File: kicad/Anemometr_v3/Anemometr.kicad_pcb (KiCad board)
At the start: 2 copper layers, 45 x 45 mm, 170 parts, among them J1 TxD, J10 +Z1, J11 +Z2, J12 +Z3, J13 +Z4, J14 -Z1, J15 -Z2, J16 -Z3, J17 -Z4, J18 1 TxD+, J19 2 TxD-, J2 RxD, J20 3 RxD+, J21 4-5, J22 6 RxD-, J23 7-8, J24 Conn_01x01_Female, J25 Conn_01x01_Female, J26 Conn_01x01_Female, J3 SCL, J4 SDA, J5 RST, J6 +EXT, J7 -EXT, J8 SWD, J9 SWC, Q1 5N10, U1 STM32F103C8Tx, U2 TS5A3166DBVR, U3 TS5A3166DBVR, U4 LMR14206, U5 TS5A3166DBVR, U6 NCP1117-3.3, U7 TS5A3166DBVR, U8 MCP1703-3.3, U9 MCP1703-3.3, Y1 CSTCE8M00G52A-R0, Y2 ECS-250-20-33

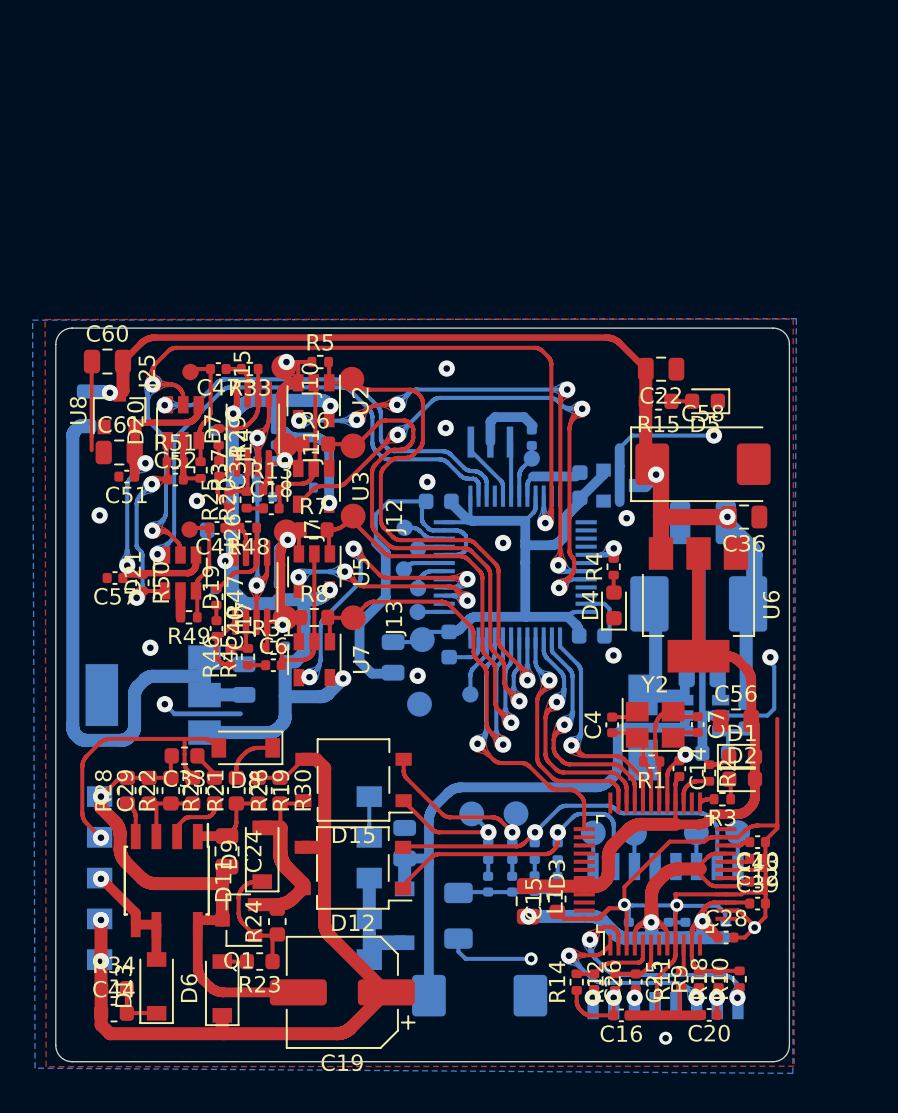
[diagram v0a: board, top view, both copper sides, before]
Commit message: изменено:      kicad/Anemometr_v3/Anemometr-cache.lib 	изменено:      kicad/Anemometr_v3/Anemometr.kicad_pcb 	изменено:      kicad/Anemometr_v3/Anemometr.kicad_pcb-bak 	изменено:      kicad/Anemometr_v3/Anemometr.sch 	изменено:      kicad/Anemometr_v3/Anemometr.sch-bak
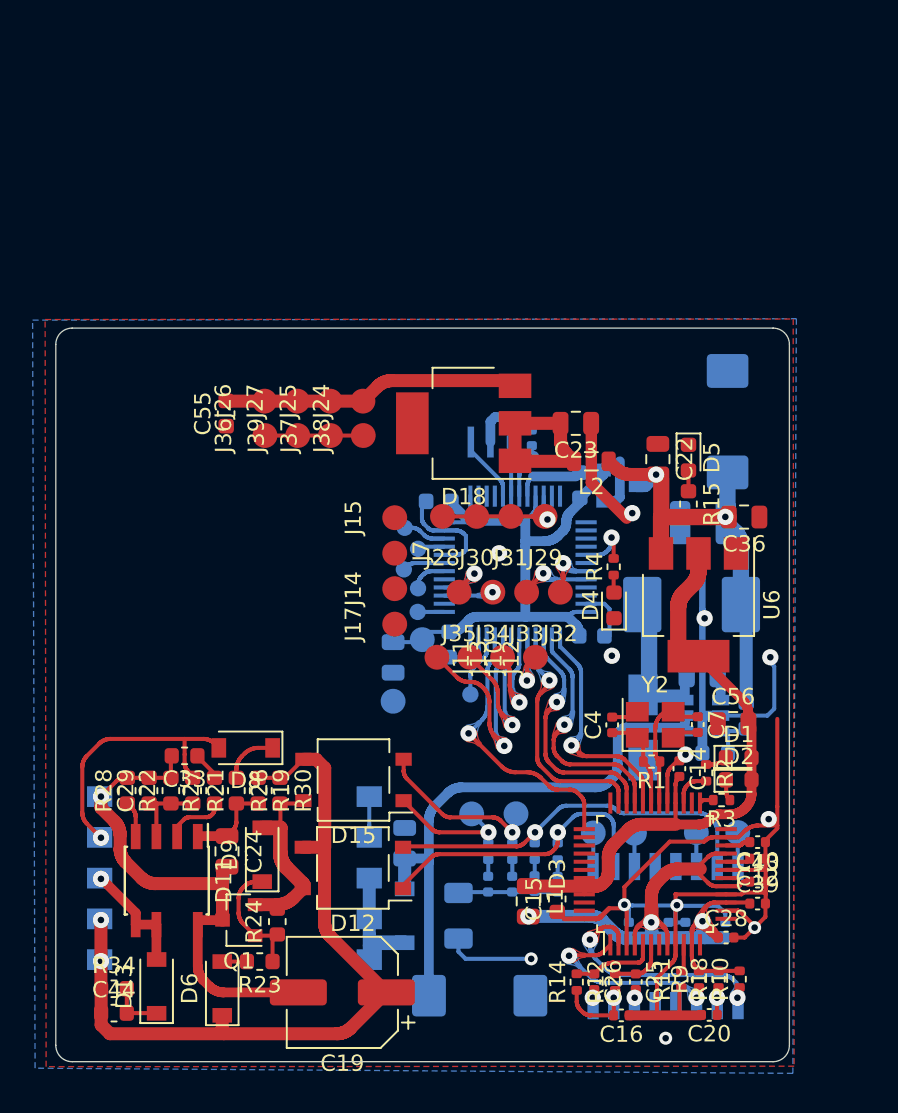
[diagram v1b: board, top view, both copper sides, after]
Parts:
- removed C1, C17, C2, C21, C32, C5, C51, C52, C57, C59: 0.1uF, Capacitor_SMD:C_0402_1005Metric
- removed C18, C6: 10nF, Capacitor_SMD:C_0402_1005Metric
- removed C34, C40: 100nF, Capacitor_SMD:C_0402_1005Metric
- removed C41, C47: 1,5nF, Capacitor_SMD:C_0402_1005Metric
- removed C60, C61: 10uF, Capacitor_SMD:C_0805_2012Metric
- removed D19, D7: MAX4477, Package_SO:MSOP-8_3x3mm_P0.65mm
- removed D20, D21: TLV3501, Package_TO_SOT_SMD:SOT-23-6
- removed R13, R31: 20k, Resistor_SMD:R_0402_1005Metric
- removed R16, R25, R33, R46, R48, R50: 100k, Resistor_SMD:R_0402_1005Metric
- removed R17: 110k, Resistor_SMD:R_0402_1005Metric
- removed R20, R45: 1k, Resistor_SMD:R_0402_1005Metric
- removed R29, R47: 5.1k, Resistor_SMD:R_0402_1005Metric
- removed R37, R49: 10k, Resistor_SMD:R_0402_1005Metric
- removed R5, R51: 3k, Resistor_SMD:R_0402_1005Metric
- removed R6, R7, R8: 3k, Resistor_SMD:R_0603_1608Metric
- removed U2, U3, U5, U7: TS5A3166DBVR, Package_TO_SOT_SMD:SOT-23-5
- removed U8: MCP1703-3.3, Package_TO_SOT_SMD:SOT-23
- added J27: +Z1, My-library:SMD-CONN, F.Cu at (33.8, 64.5)
- added J28: +Z1, My-library:SMD-CONN, F.Cu at (42.7, 71.5)
- added J29: +Z1, My-library:SMD-CONN, F.Cu at (49.0, 71.5)
- added J30: +Z1, My-library:SMD-CONN, F.Cu at (44.8, 71.5)
- added J31: +Z1, My-library:SMD-CONN, F.Cu at (46.9, 71.5)
- added J32: +Z1, My-library:SMD-CONN, F.Cu at (50.0, 76.2)
- added J33: +Z1, My-library:SMD-CONN, F.Cu at (47.9, 76.2)
- added J34: +Z1, My-library:SMD-CONN, F.Cu at (45.8, 76.2)
- added J35: +Z1, My-library:SMD-CONN, F.Cu at (43.7, 76.2)
- added J36: +Z1, My-library:SMD-CONN, F.Cu at (31.8, 66.6)
- added J37: +Z1, My-library:SMD-CONN, F.Cu at (35.9, 66.6)
- added J38: +Z1, My-library:SMD-CONN, F.Cu at (37.9, 66.6)
- added J39: +Z1, My-library:SMD-CONN, F.Cu at (33.8, 66.6)
- C23, C55, D18, L2: moved to F.Cu
- C58: moved to B.Cu
- D11: value SD4932B -> U6119SA
- J24: value Conn_01x01_Female -> +Z1; footprint My-library:ConnMini -> My-library:SMD-CONN; moved to F.Cu
- J25, J26: value Conn_01x01_Female -> +Z1; footprint My-library:ConnMini -> My-library:SMD-CONN
- moved L2 31.1 mm to (51.9, 68.2), turned to 180 degrees
- moved C23 25.7 mm to (50.9, 65.8), turned to 180 degrees
- moved D18 25.3 mm to (44.0, 65.8)
- moved J10 20.4 mm to (48.4, 80.2)
- moved J11 15.9 mm to (46.4, 80.2)
- moved J24 12.8 mm to (37.8, 64.5), turned to 270 degrees
- moved J15 11.5 mm to (39.8, 71.6)
- moved J12 11.2 mm to (44.4, 80.2)
- moved J14 11.1 mm to (39.8, 76.0)
- moved J26 9.12 mm to (31.8, 64.5), turned to 270 degrees
- moved J25 8.73 mm to (35.8, 64.5)
- moved C55 7.17 mm to (29.4, 65.2), turned to 90 degrees
- moved J7 6.78 mm to (39.8, 73.8)
- moved J17 6.73 mm to (39.8, 78.2)
- moved R15 6.57 mm to (57.8, 70.8), turned to 270 degrees
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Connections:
- J24 pad 1: SInput -> +5VA
- J25 pad 1: Net-(C47-Pad2) -> +5VA
- J26 pad 1: Net-(C41-Pad2) -> +5VA
- U1 pad 10: SInput -> SIn
- U1 pad 19: Z1 -> Z1Sel
- U1 pad 2: Z3-4 -> (no net)
- U1 pad 20: Z2 -> Z2Sel
- U1 pad 3: Z1-2 -> (no net)
- U1 pad 39: Z3 -> Z3Sel
- U1 pad 40: Z4 -> Z4Sel
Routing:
- net SInput: track 53.4 -> 0.00 mm, vias 3 -> 0
- net GND: track 192.9 -> 139.8 mm, vias 23 -> 12
- net 6v: track 67.2 -> 27.6 mm, vias 3 -> 2
- net +5VA: track 54.6 -> 18.3 mm, vias 6 -> 0
- net Z2: track 33.9 -> 0.00 mm, vias 3 -> 0
- net Z3-4: track 32.1 -> 0.00 mm, vias 1 -> 0
- net /+Z1: track 35.2 -> 4.27 mm
- net Z1: track 30.0 -> 0.00 mm, vias 5 -> 0
- net /+Z2: track 36.2 -> 7.30 mm
- net Z1-2: track 24.9 -> 0.00 mm, vias 1 -> 0
- net Net-(C23-Pad2): track 35.3 -> 11.3 mm
- net +3.3VP: track 21.4 -> 0.00 mm, vias 2 -> 0
- net Z4: track 19.2 -> 0.00 mm, vias 3 -> 0
- net a: track 18.5 -> 0.00 mm, vias 2 -> 0
- net /+Z3: track 28.1 -> 10.7 mm
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
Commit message: изменено:      kicad/Anemometr_v3/Anemometr.kicad_pcb 	изменено:      kicad/Anemometr_v3/Anemometr.kicad_pcb-bak 	изменено:      stm32cubeide/Anemometr_v3/Anemometr_3.ioc 	изменено:      stm32cubeide/Anemometr_v3/Core/Inc/main.h 	изменено:      stm32cubeide/Anemometr_v3/Core/Src/main.c 	изменено:      stm32cubeide/Anemometr_v3/Core/Src/stm32f1xx_hal_msp.c 	изменено:      stm32cubeide/Anemometr_v3/Debug/Anemometr_3.bin 	изменено:      stm32cubeide/Anemometr_v3/Debug/Anemometr_3.elf 	изменено:      stm32cubeide/Anemometr_v3/Debug/Anemometr_3.list 	изменено:      stm32cubeide/Anemometr_v3/Debug/Anemometr_3.map 	изменено:      stm32cubeide/Anemometr_v3/Debug/Core/Src/BME280.o 	изменено:      stm32cubeide/Anemometr_v3/Debug/Core/Src/main.o 	изменено:      stm32cubeide/Anemometr_v3/Debug/Core/Src/main.su 	изменено:      stm32cubeide/Anemometr_v3/Debug/Core/Src/stm32f1xx_hal_msp.o 	изменено:      stm32cubeide/Anemometr_v3/Debug/Core/Src/stm32f1xx_it.o
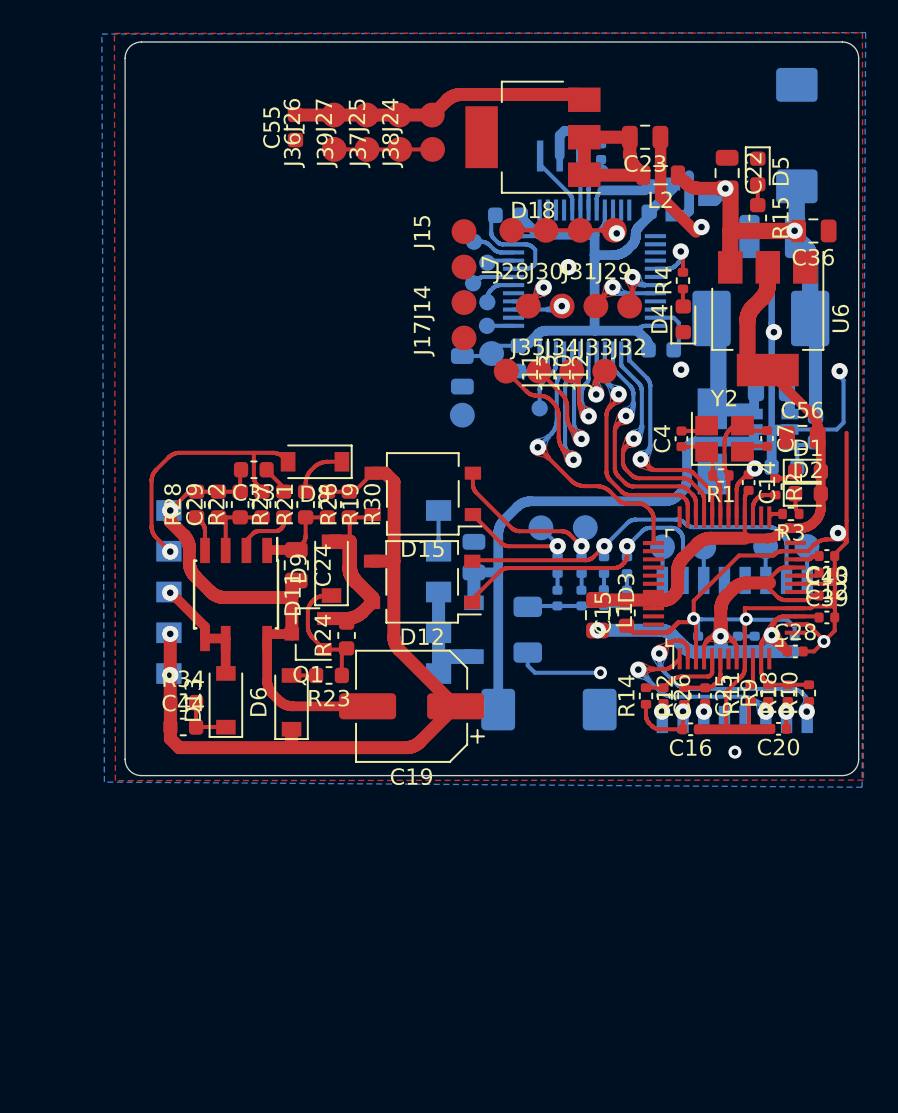
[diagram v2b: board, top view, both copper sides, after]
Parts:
- moved C14 18.1 mm to (61.5, 69.5)
- moved C27 18.1 mm to (61.9, 79.4)
- moved C35 18.1 mm to (58.4, 79.4)
- moved C38 18.1 mm to (60.8, 79.4)
- moved C45 18.1 mm to (52.6, 76.5)
- moved C56 18.1 mm to (64.8, 66.7)
- moved D10 18.1 mm to (60.7, 79.7)
- moved D15 18.1 mm to (41.5, 70.2)
- moved J21 18.1 mm to (51.5, 72.2)
- moved L1 18.1 mm to (52.2, 77.6)
- moved R23 18.1 mm to (35.8, 81.3)
- moved R34 18.1 mm to (26.8, 83.0)
- moved C22 18.1 mm to (60.2, 50.5)
- moved C23 18.1 mm to (55.1, 48.3)
- moved C3 18.1 mm to (52.5, 49.2)
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
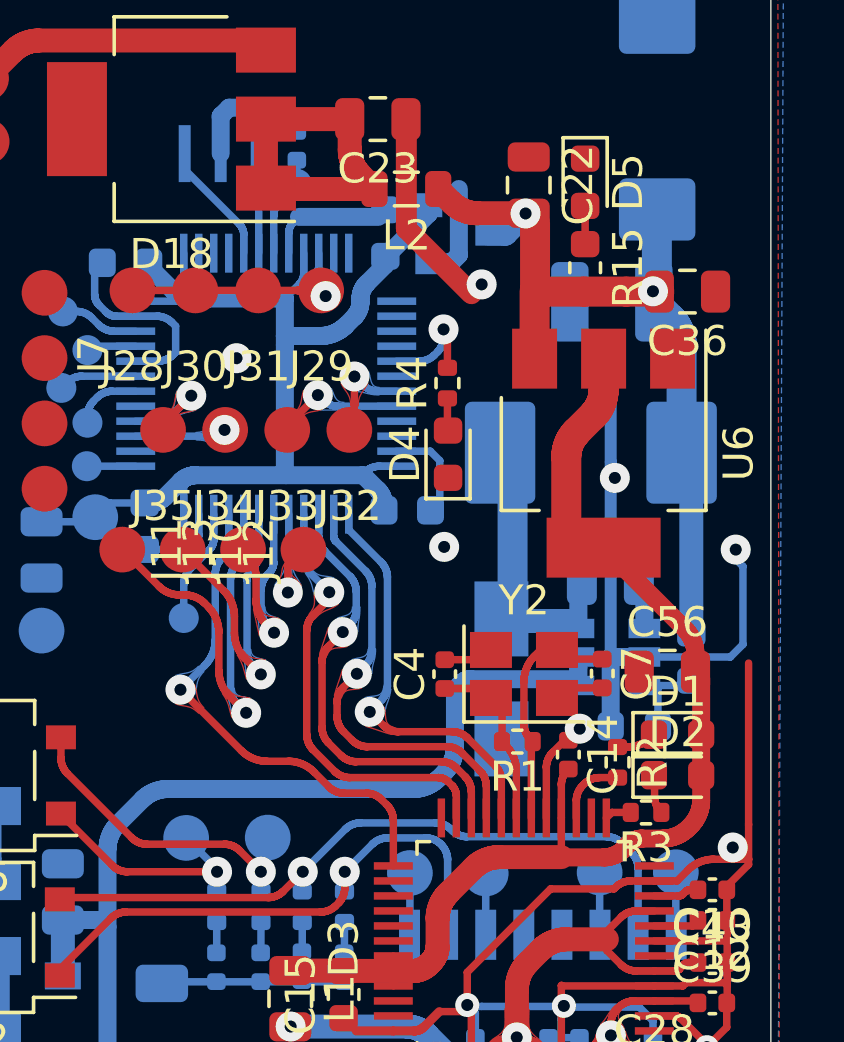
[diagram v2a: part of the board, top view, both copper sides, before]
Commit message: изменено:      kicad/Anemometr_v3/Anemometr.kicad_pcb 	изменено:      kicad/Anemometr_v3/Anemometr.kicad_pcb-bak
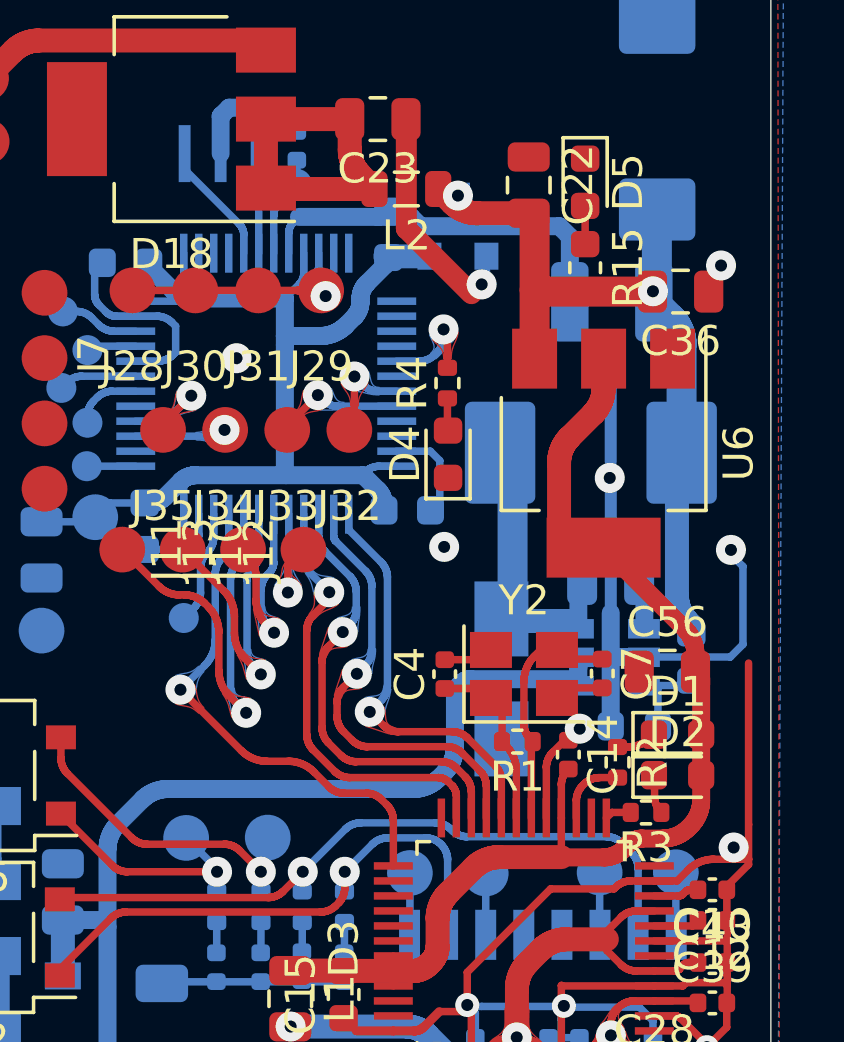
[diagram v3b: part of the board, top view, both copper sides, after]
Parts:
- moved U9 0.25 mm to (57.8, 51.9), turned to 90 degrees
- moved C36 0.23 mm to (65.2, 54.0)
- moved C9 0.11 mm to (55.5, 52.1)
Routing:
- net GND: track 139.8 -> 145.5 mm, vias 12 -> 13
- net +3V3: track 38.1 -> 37.3 mm
